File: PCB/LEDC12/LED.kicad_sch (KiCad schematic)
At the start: 38 parts, among them J1 Reset, J2 Wago, J3 USB-C-Socket-H, J4 TC2030-USB-NL-DS, SW1 Button, U1 ESP32-S3-MINI-1, U2 IRMHF384, U3 ICS43434_MEMS_Mic, U4 TPS562243

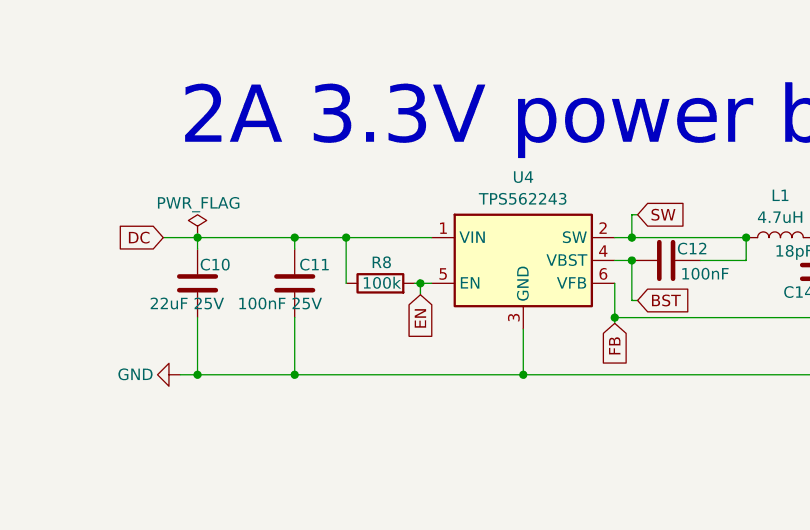
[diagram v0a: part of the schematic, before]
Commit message: Margins tidy
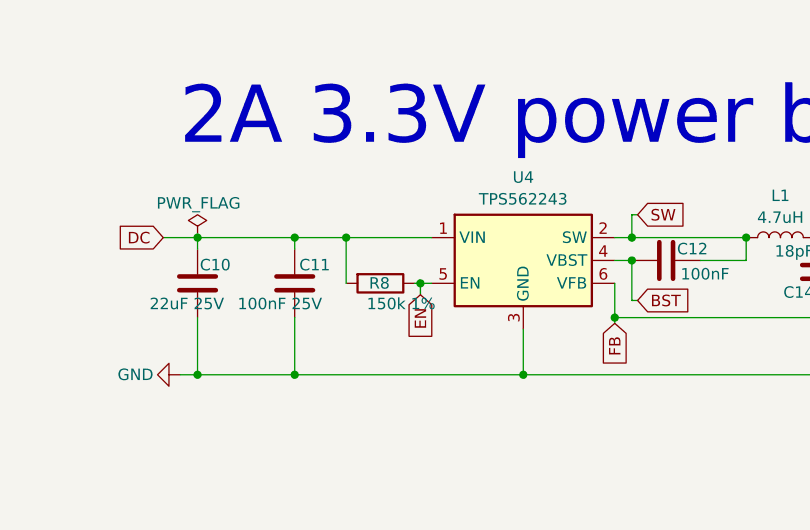
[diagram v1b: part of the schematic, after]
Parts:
- R8: value 100k -> 150k 1%; MPN C106224 -> C310173
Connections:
- net DC: now also R8.2; no longer R8.1
- net EN: now also R8.1; no longer R8.2
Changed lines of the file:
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@@
+	)
+	(symbol
+		(lib_id "Device:R")
+		(at 207.01 152.4 270)
+		(unit 1)
+		(exclude_from_sim no)
+		(in_bom yes)
+		(on_board yes)
+		(dnp no)
+		(property "Reference" "R8"
+			(at 205.74 152.4 90)
+			(effects
+				(font
+					(size 1.27 1.27)
+				)
+				(justify left)
+			)
+		)
+		(property "Value" "150k 1%"
+			(at 205.486 154.686 90)
+			(effects
+				(font
+					(size 1.27 1.27)
+				)
+				(justify left)
+			)
+		)
+		(property "Footprint" "RevK:R_0201"
+			(at 207.01 150.622 90)
+			(effects
+				(font
+					(size 1.27 1.27)
+				)
+				(hide yes)
+			)
+		)
+		(property "Datasheet" "~"
+			(at 207.01 152.4 0)
+			(effects
+				(font
+					(size 1.27 1.27)
+				)
+				(hide yes)
+			)
+		)
+		(property "Description" "Resistor"
+			(at 207.01 152.4 0)
+			(effects
+				(font
+					(size 1.27 1.27)
+				)
+				(hide yes)
+			)
+		)
+		(property "MPN" "C310173"
+			(at 207.01 152.4 0)
+			(effects
+				(font
+					(size 1.27 1.27)
+				)
+				(hide yes)
+			)
+		)
+		(pin "1"
+		)
+		(pin "2"
+		)
+		(instances
+			(project "LED"
+				(path "/46c350bb-7de4-4e81-aafd-4af55e37aab0"
+					(reference "R8")
+					(unit 1)
+				)
+			)
+		)
 	)
 	(symbol
@@
 					(unit 1)
 				)
-			)
-		)
-	)
-	(symbol
-		(lib_id "Device:R")
-		(at 207.01 152.4 90)
-		(unit 1)
-		(exclude_from_sim no)
-		(in_bom yes)
-		(on_board yes)
-		(dnp no)
-		(property "Reference" "R8"
-			(at 207.137 150.114 90)
-			(effects
-				(font
-					(size 1.27 1.27)
-				)
-			)
-		)
-		(property "Value" "100k"
-			(at 207.137 152.4 90)
-			(effects
-				(font
-					(size 1.27 1.27)
-				)
-			)
-		)
-		(property "Footprint" "RevK:R_0201"
-			(at 207.01 154.178 90)
-			(effects
-				(font
-					(size 1.27 1.27)
-				)
-				(hide yes)
-			)
-		)
-		(property "Datasheet" "~"
-			(at 207.01 152.4 0)
-			(effects
-				(font
-					(size 1.27 1.27)
-				)
-				(hide yes)
-			)
-		)
-		(property "Description" "Resistor"
-			(at 207.01 152.4 0)
-			(effects
-				(font
-					(size 1.27 1.27)
-				)
-				(hide yes)
-			)
-		)
-		(property "MPN" "C106224"
-			(at 207.01 152.4 90)
-			(effects
-				(font
-					(size 1.27 1.27)
-				)
-				(hide yes)
-			)
-		)
-		(pin "1"
-		)
-		(pin "2"
-		)
-		(instances
-			(project "LED"
-				(path "/46c350bb-7de4-4e81-aafd-4af55e37aab0"
-					(reference "R8")
-					(unit 1)
-				)
